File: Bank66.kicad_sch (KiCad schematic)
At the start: 1 part, among them U1 XCKU5P-FFVB676

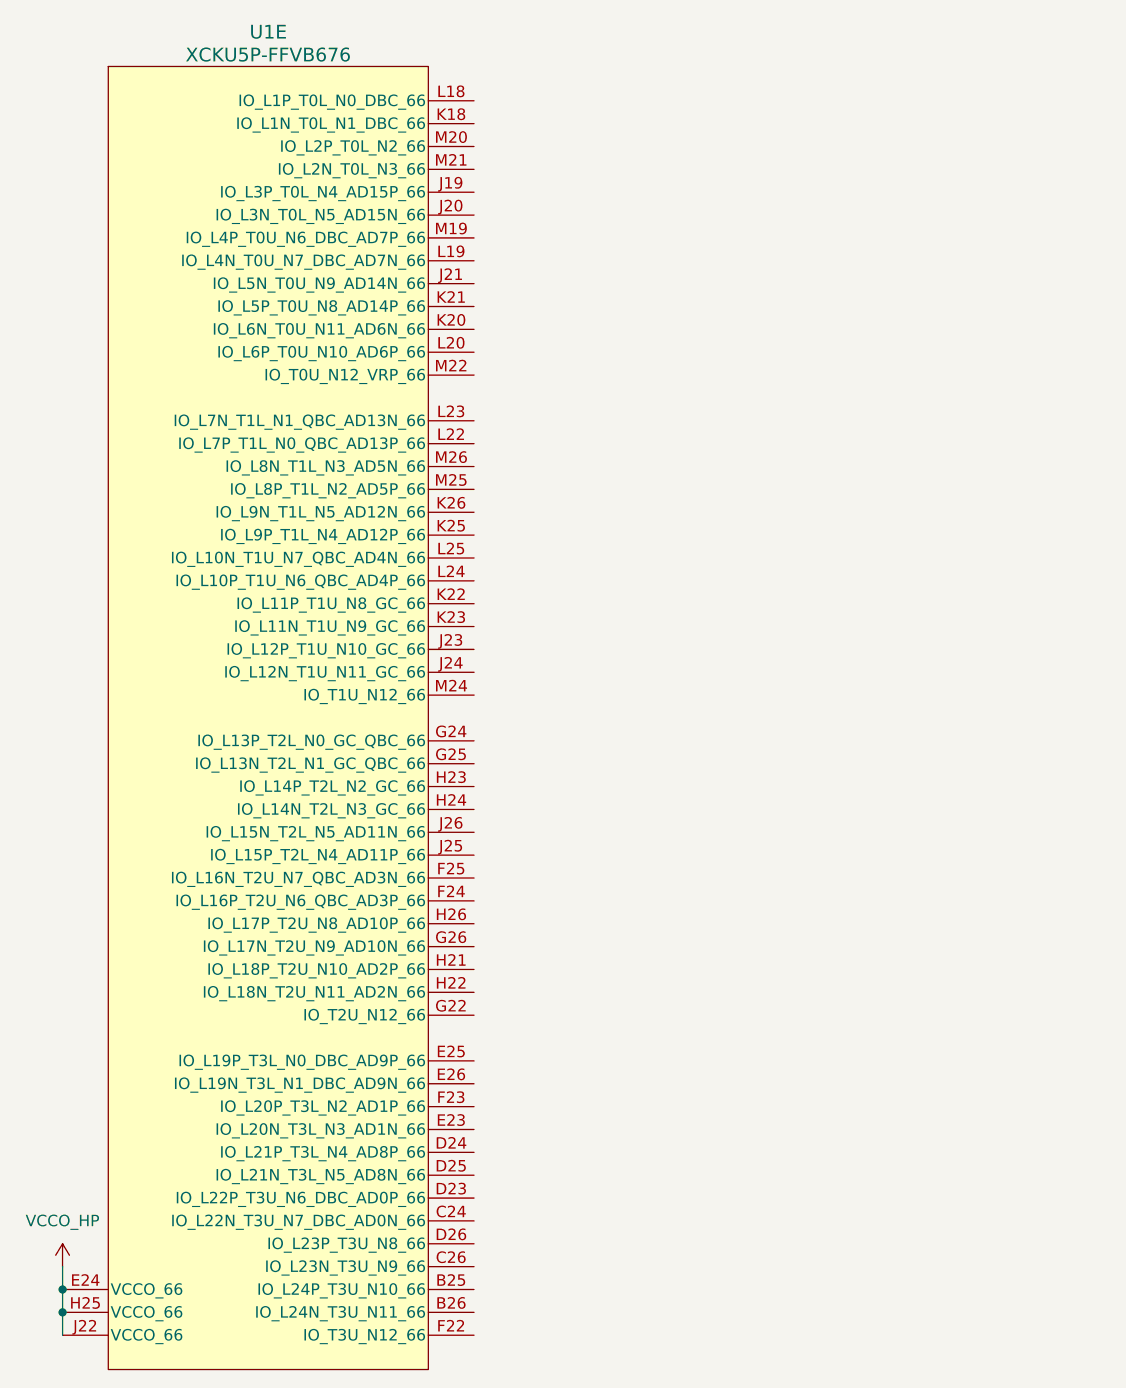
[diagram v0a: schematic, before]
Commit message: finishing schematic
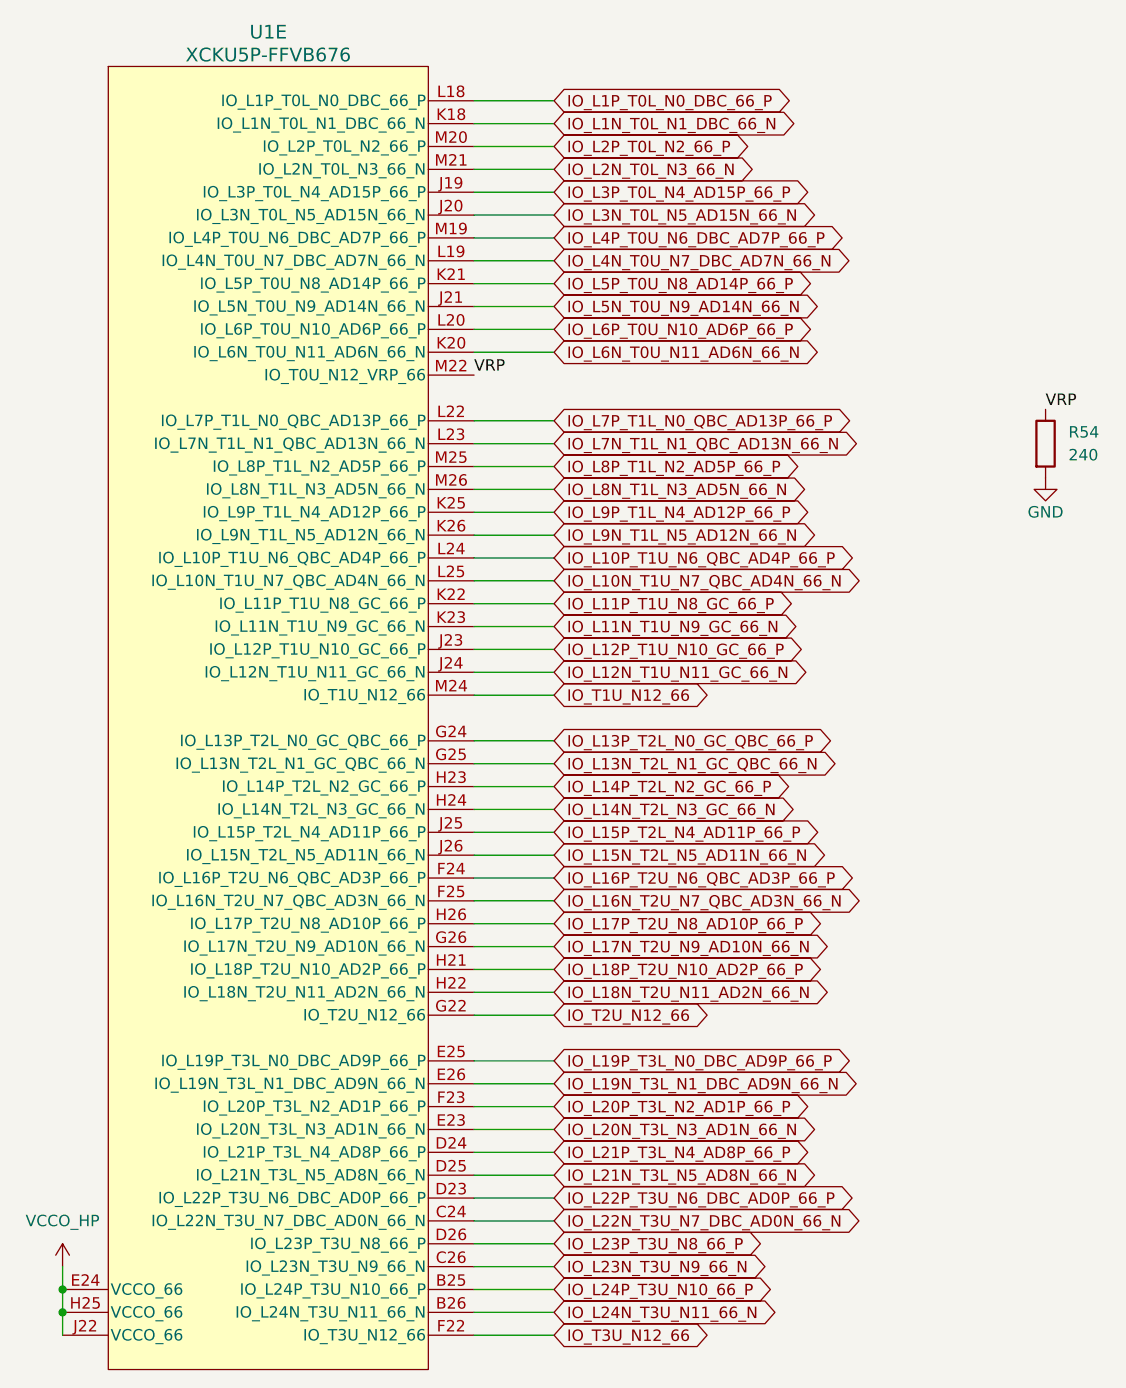
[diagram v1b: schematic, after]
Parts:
- added R54: 240, Resistor_SMD:R_0201_0603Metric, symbol Device:R
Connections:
- net IO_L24P_T3U_N10_66_P: now reaches U1.B25 (IO_L24P_T3U_N10_66_P)
- net IO_L24N_T3U_N11_66_N: now reaches U1.B26 (IO_L24N_T3U_N11_66_N)
- net IO_L22N_T3U_N7_DBC_AD0N_66_N: now reaches U1.C24 (IO_L22N_T3U_N7_DBC_AD0N_66_N)
- net IO_L23N_T3U_N9_66_N: now reaches U1.C26 (IO_L23N_T3U_N9_66_N)
- net IO_L22P_T3U_N6_DBC_AD0P_66_P: now reaches U1.D23 (IO_L22P_T3U_N6_DBC_AD0P_66_P)
- net IO_L21P_T3L_N4_AD8P_66_P: now reaches U1.D24 (IO_L21P_T3L_N4_AD8P_66_P)
- net IO_L21N_T3L_N5_AD8N_66_N: now reaches U1.D25 (IO_L21N_T3L_N5_AD8N_66_N)
- net IO_L23P_T3U_N8_66_P: now reaches U1.D26 (IO_L23P_T3U_N8_66_P)
- net IO_L20N_T3L_N3_AD1N_66_N: now reaches U1.E23 (IO_L20N_T3L_N3_AD1N_66_N)
- net IO_L19P_T3L_N0_DBC_AD9P_66_P: now reaches U1.E25 (IO_L19P_T3L_N0_DBC_AD9P_66_P)
- net IO_L19N_T3L_N1_DBC_AD9N_66_N: now reaches U1.E26 (IO_L19N_T3L_N1_DBC_AD9N_66_N)
- net IO_T3U_N12_66: now reaches U1.F22 (IO_T3U_N12_66)
- net IO_L20P_T3L_N2_AD1P_66_P: now reaches U1.F23 (IO_L20P_T3L_N2_AD1P_66_P)
- net IO_L16P_T2U_N6_QBC_AD3P_66_P: now reaches U1.F24 (IO_L16P_T2U_N6_QBC_AD3P_66_P)
- net IO_L16N_T2U_N7_QBC_AD3N_66_N: now reaches U1.F25 (IO_L16N_T2U_N7_QBC_AD3N_66_N)
- net IO_T2U_N12_66: now reaches U1.G22 (IO_T2U_N12_66)
- net IO_L13P_T2L_N0_GC_QBC_66_P: now reaches U1.G24 (IO_L13P_T2L_N0_GC_QBC_66_P)
- net IO_L13N_T2L_N1_GC_QBC_66_N: now reaches U1.G25 (IO_L13N_T2L_N1_GC_QBC_66_N)
- net IO_L17N_T2U_N9_AD10N_66_N: now reaches U1.G26 (IO_L17N_T2U_N9_AD10N_66_N)
- net IO_L18P_T2U_N10_AD2P_66_P: now reaches U1.H21 (IO_L18P_T2U_N10_AD2P_66_P)
- net IO_L18N_T2U_N11_AD2N_66_N: now reaches U1.H22 (IO_L18N_T2U_N11_AD2N_66_N)
- net IO_L14P_T2L_N2_GC_66_P: now reaches U1.H23 (IO_L14P_T2L_N2_GC_66_P)
- net IO_L14N_T2L_N3_GC_66_N: now reaches U1.H24 (IO_L14N_T2L_N3_GC_66_N)
- net IO_L17P_T2U_N8_AD10P_66_P: now reaches U1.H26 (IO_L17P_T2U_N8_AD10P_66_P)
- net IO_L3P_T0L_N4_AD15P_66_P: now reaches U1.J19 (IO_L3P_T0L_N4_AD15P_66_P)
- net IO_L3N_T0L_N5_AD15N_66_N: now reaches U1.J20 (IO_L3N_T0L_N5_AD15N_66_N)
- net IO_L5N_T0U_N9_AD14N_66_N: now reaches U1.J21 (IO_L5N_T0U_N9_AD14N_66_N)
- net IO_L12P_T1U_N10_GC_66_P: now reaches U1.J23 (IO_L12P_T1U_N10_GC_66_P)
- net IO_L12N_T1U_N11_GC_66_N: now reaches U1.J24 (IO_L12N_T1U_N11_GC_66_N)
- net IO_L15P_T2L_N4_AD11P_66_P: now reaches U1.J25 (IO_L15P_T2L_N4_AD11P_66_P)
- net IO_L15N_T2L_N5_AD11N_66_N: now reaches U1.J26 (IO_L15N_T2L_N5_AD11N_66_N)
- net IO_L1N_T0L_N1_DBC_66_N: now reaches U1.K18 (IO_L1N_T0L_N1_DBC_66_N)
- net IO_L6N_T0U_N11_AD6N_66_N: now reaches U1.K20 (IO_L6N_T0U_N11_AD6N_66_N)
- net IO_L5P_T0U_N8_AD14P_66_P: now reaches U1.K21 (IO_L5P_T0U_N8_AD14P_66_P)
- net IO_L11P_T1U_N8_GC_66_P: now reaches U1.K22 (IO_L11P_T1U_N8_GC_66_P)
- net IO_L11N_T1U_N9_GC_66_N: now reaches U1.K23 (IO_L11N_T1U_N9_GC_66_N)
- net IO_L9P_T1L_N4_AD12P_66_P: now reaches U1.K25 (IO_L9P_T1L_N4_AD12P_66_P)
- net IO_L9N_T1L_N5_AD12N_66_N: now reaches U1.K26 (IO_L9N_T1L_N5_AD12N_66_N)
- net IO_L1P_T0L_N0_DBC_66_P: now reaches U1.L18 (IO_L1P_T0L_N0_DBC_66_P)
- net IO_L4N_T0U_N7_DBC_AD7N_66_N: now reaches U1.L19 (IO_L4N_T0U_N7_DBC_AD7N_66_N)
- net IO_L6P_T0U_N10_AD6P_66_P: now reaches U1.L20 (IO_L6P_T0U_N10_AD6P_66_P)
- net IO_L7P_T1L_N0_QBC_AD13P_66_P: now reaches U1.L22 (IO_L7P_T1L_N0_QBC_AD13P_66_P)
- net IO_L7N_T1L_N1_QBC_AD13N_66_N: now reaches U1.L23 (IO_L7N_T1L_N1_QBC_AD13N_66_N)
- net IO_L10P_T1U_N6_QBC_AD4P_66_P: now reaches U1.L24 (IO_L10P_T1U_N6_QBC_AD4P_66_P)
- net IO_L10N_T1U_N7_QBC_AD4N_66_N: now reaches U1.L25 (IO_L10N_T1U_N7_QBC_AD4N_66_N)
- net IO_L4P_T0U_N6_DBC_AD7P_66_P: now reaches U1.M19 (IO_L4P_T0U_N6_DBC_AD7P_66_P)
- net IO_L2P_T0L_N2_66_P: now reaches U1.M20 (IO_L2P_T0L_N2_66_P)
- net IO_L2N_T0L_N3_66_N: now reaches U1.M21 (IO_L2N_T0L_N3_66_N)
- net VRP: now reaches U1.M22 (IO_T0U_N12_VRP_66)
- net VRP: now also R54.1
- net IO_T1U_N12_66: now reaches U1.M24 (IO_T1U_N12_66)
- net IO_L8P_T1L_N2_AD5P_66_P: now reaches U1.M25 (IO_L8P_T1L_N2_AD5P_66_P)
- net IO_L8N_T1L_N3_AD5N_66_N: now reaches U1.M26 (IO_L8N_T1L_N3_AD5N_66_N)
- new net GND: R54.2
